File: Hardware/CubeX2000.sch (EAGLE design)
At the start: 123 parts, among them IC1 MEGA32-A, IC10 MAX232, IC2 74HC595D, IC3 74HC595D, IC4 74HC595D, IC5 74HC595D, IC6 74HC595D, IC7 74HC595D, IC8 74HC595D, IC9 74HC595D, Q1 16MHz

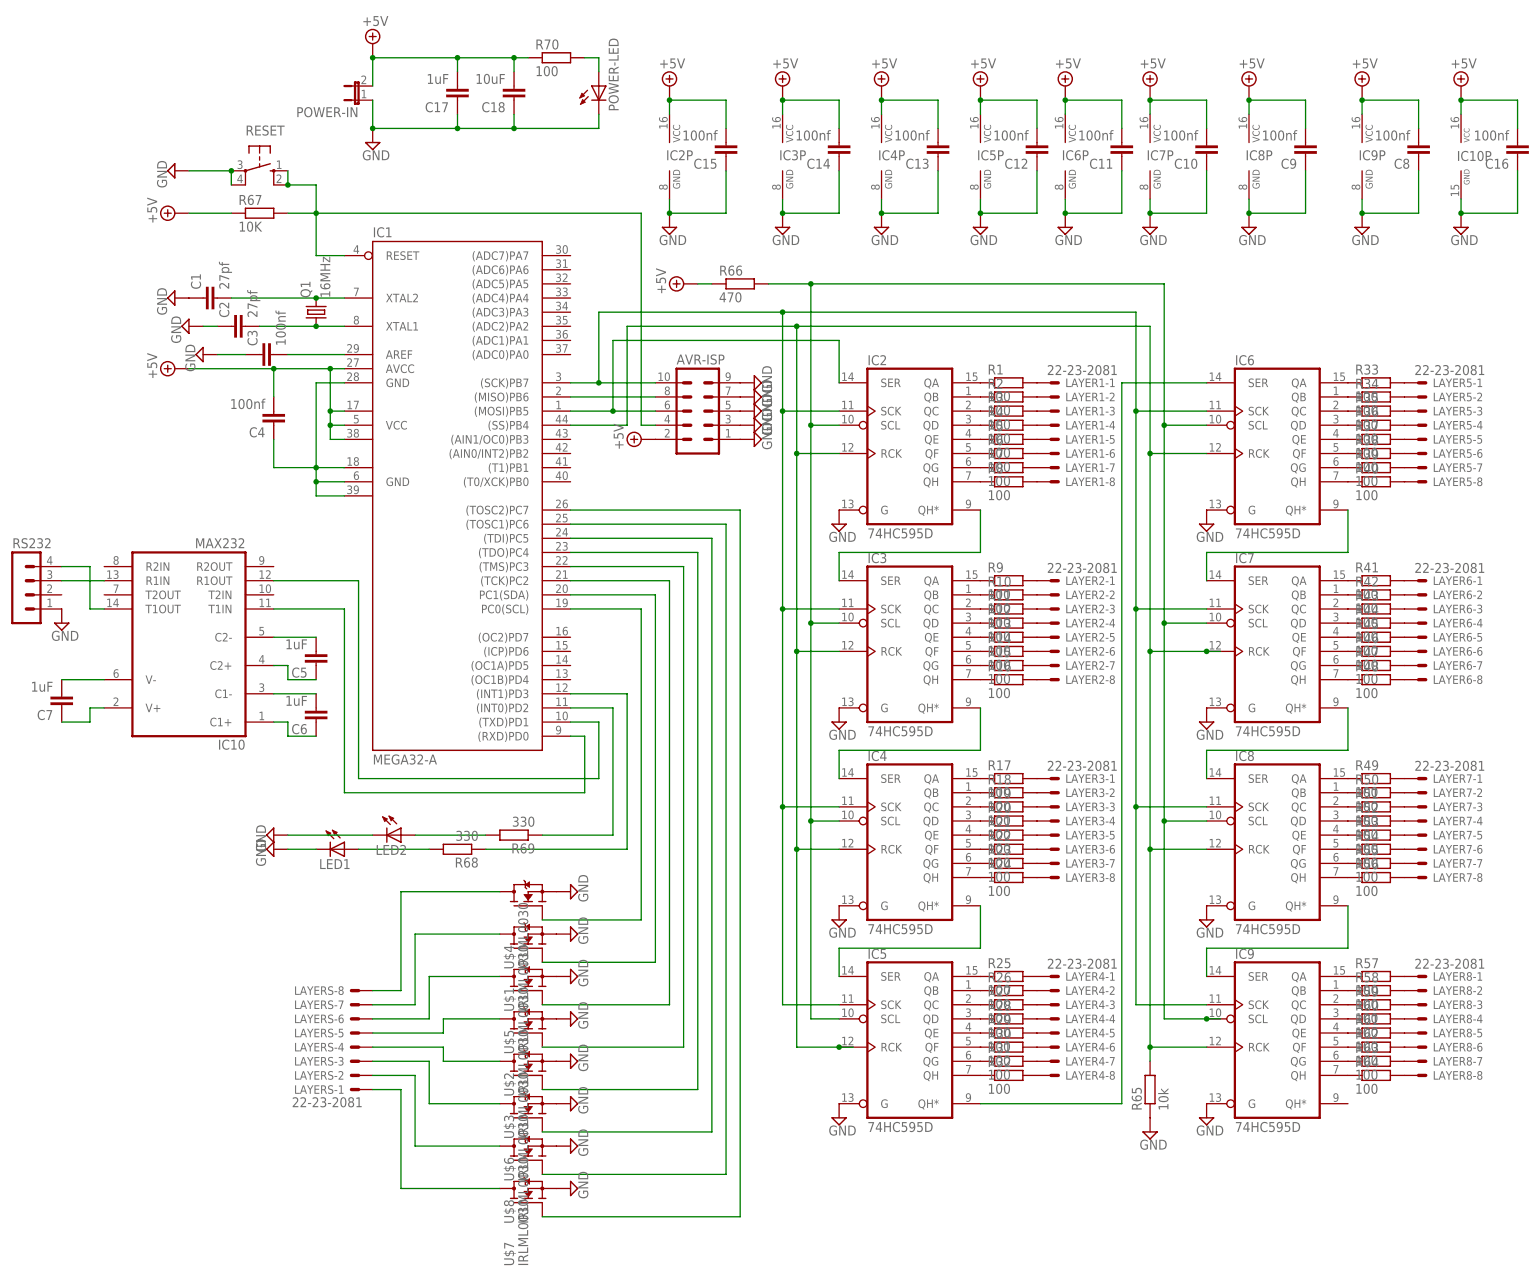
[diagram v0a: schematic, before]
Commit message: Add files via upload
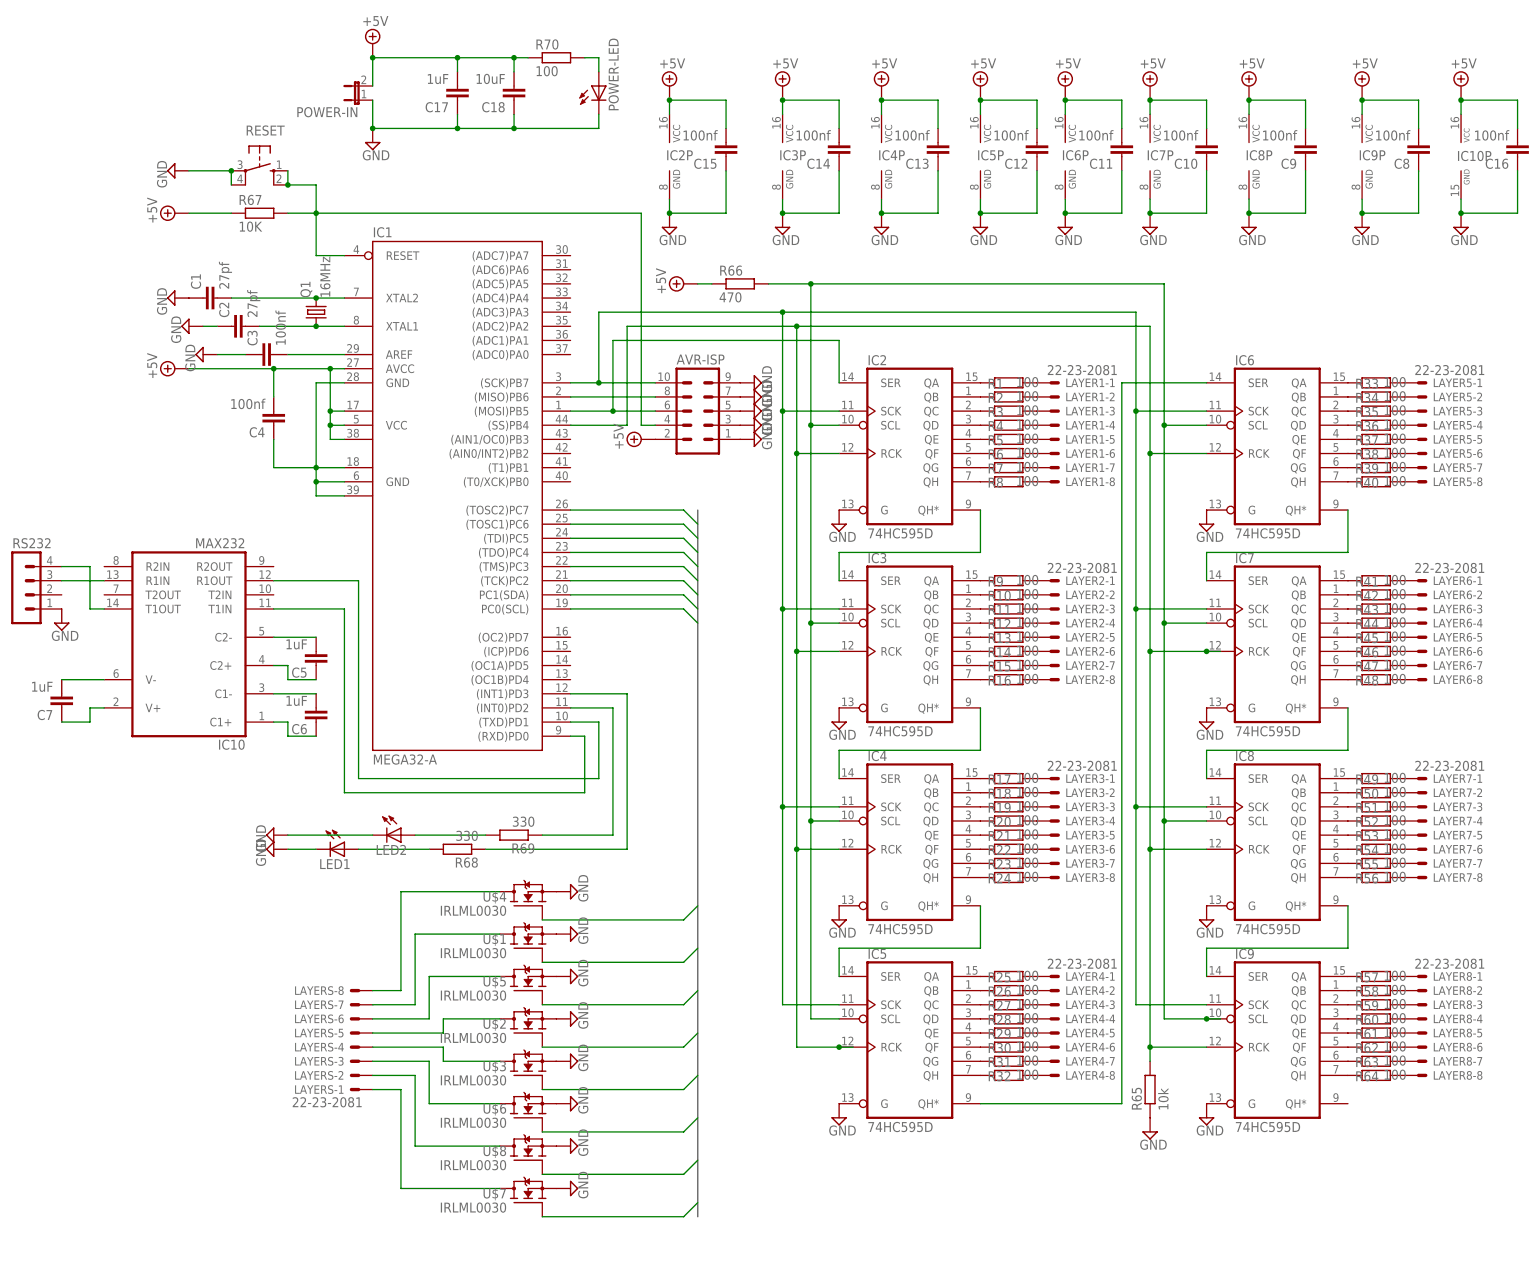
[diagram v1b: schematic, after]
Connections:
- removed net N$142: IC1.PC0(SCL), U$4.G
- removed net N$143: IC1.PC1(SDA), U$1.G
- removed net N$144: IC1.(TCK)PC2, U$5.G
- removed net N$145: IC1.(TMS)PC3, U$2.G
- removed net N$146: IC1.(TDO)PC4, U$3.G
- removed net N$147: U$6.G
- removed net N$148: IC1.(TOSC1)PC6, U$8.G
- removed net N$149: IC1.(TOSC2)PC7, U$7.G
- new net LAYERS1: IC1.PC0(SCL), U$7.G
- new net LAYERS2: IC1.PC1(SDA), U$8.G
- new net LAYERS3: IC1.(TCK)PC2, U$6.G
- new net LAYERS4: IC1.(TMS)PC3, U$3.G
- new net LAYERS5: IC1.(TDO)PC4, U$2.G
- new net LAYERS6: IC1.(TDI)PC5, U$5.G
- new net LAYERS7: IC1.(TOSC1)PC6, U$1.G
- new net LAYERS8: IC1.(TOSC2)PC7, U$4.G
